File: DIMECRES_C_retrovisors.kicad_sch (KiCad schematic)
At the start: 65 parts, among them J10 Vbat, J2 DE9_Pins, J3 Conn_01x05_Pin, J4 Motor3, J6 Intermitente, J7 Calentador, J8 Motor2, J9 Motor1, Q1 DTC144E, Q2 DTC144E, Q3 DTC144E, SW1 SW_DPDT_G6S, U2 LM1117DT-ADJ, U3 LM2596S-ADJ, U4 L298N, U5 TJA1042T, U6 ADA4511-2, U7 PIC18F4480-IP, Y1 Crystal

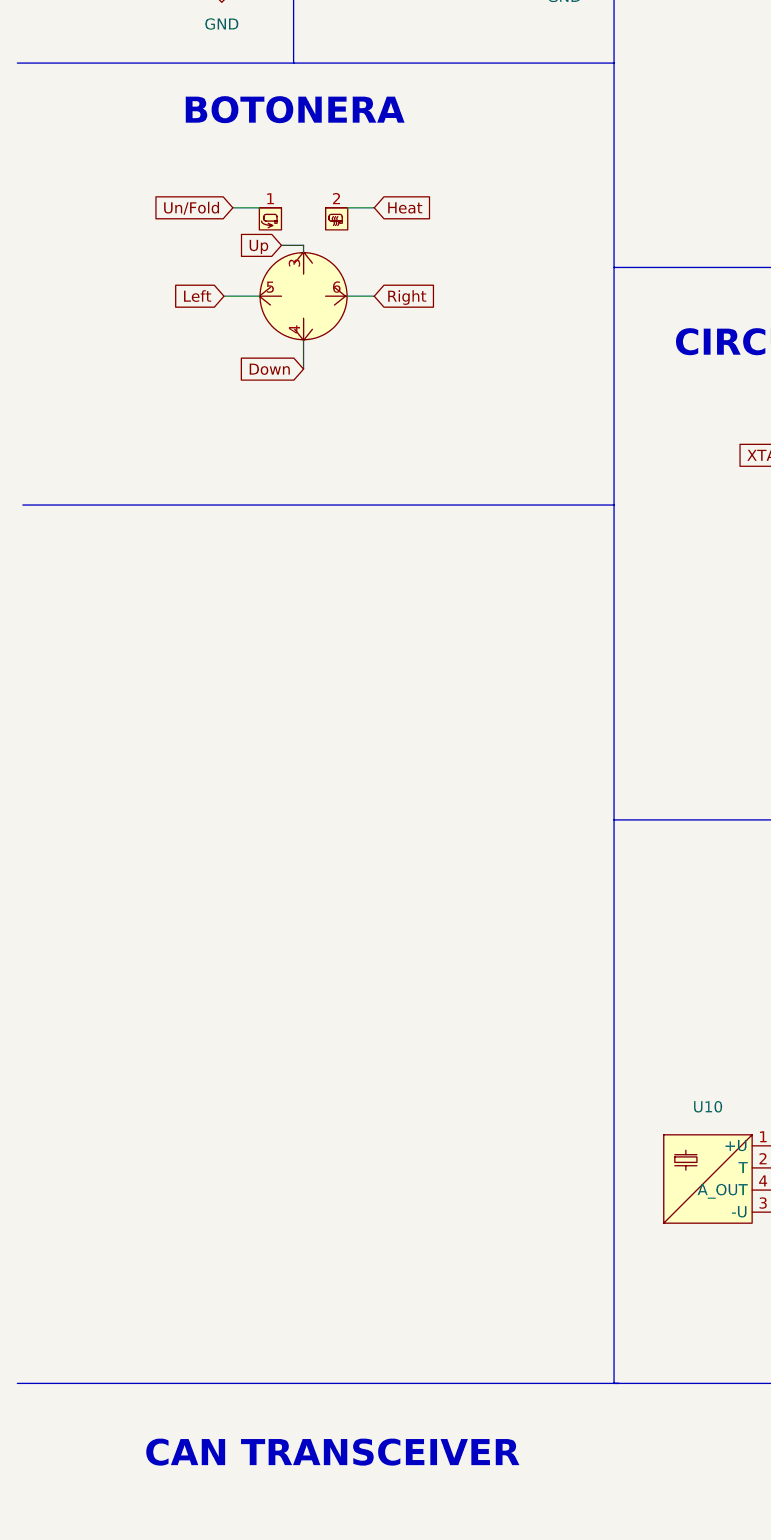
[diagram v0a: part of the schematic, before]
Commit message: Update DIMECRES_C_retrovisors.kicad_sch
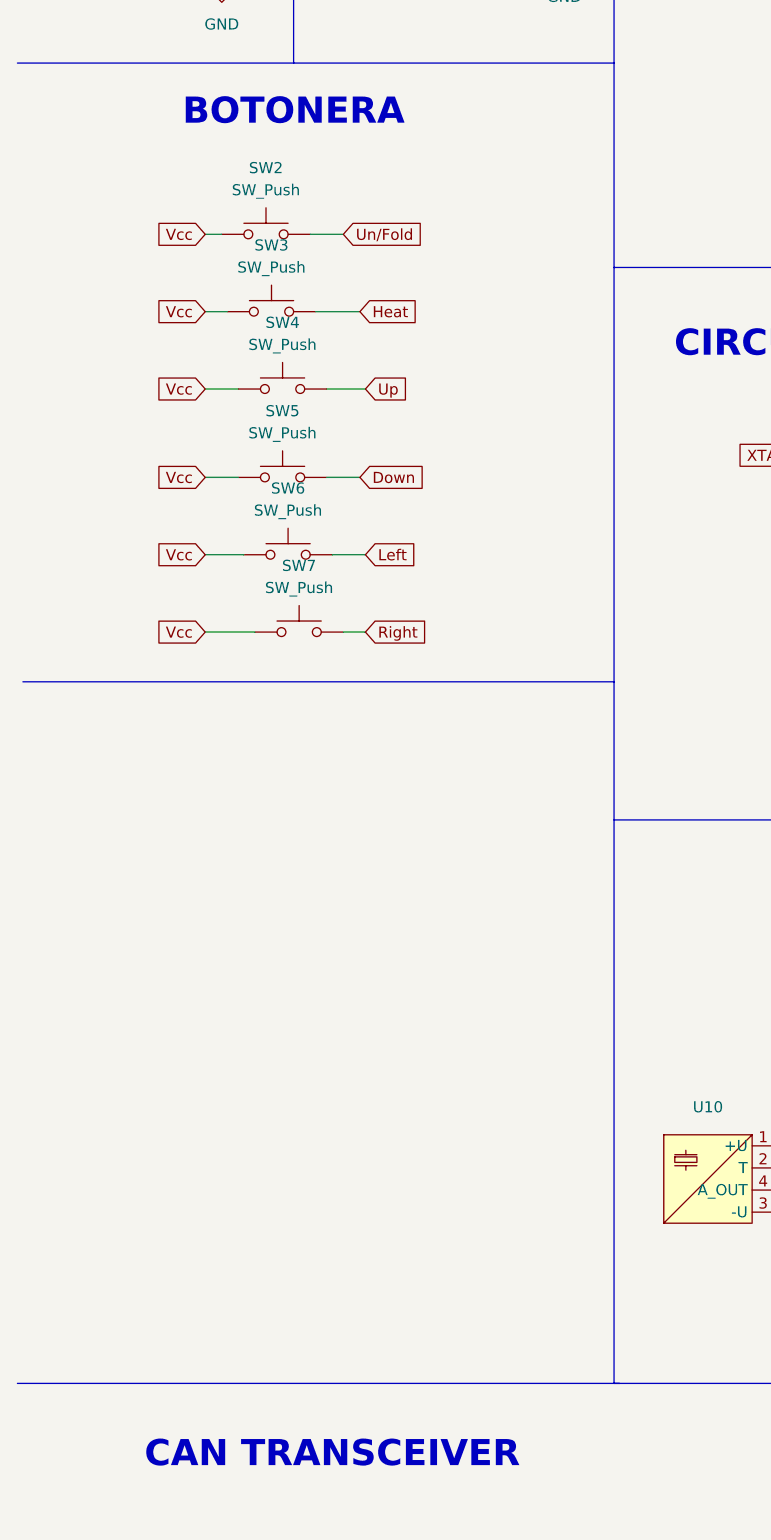
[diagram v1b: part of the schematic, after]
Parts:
- removed U1: ~, symbol PracticasKiCad:Botonera_Retrovisor
- added SW2, SW3, SW4, SW5, SW6, SW7: SW_Push, symbol Switch:SW_Push
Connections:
- net Down: now also SW5.2
- net Heat: now also SW3.2
- net Left: now also SW6.2
- net Right: now also SW7.2
- net Un/Fold: now also SW2.2
- net Up: now also SW4.2
- net Vcc: now also SW2.1, SW3.1, SW4.1, SW5.1, SW6.1, SW7.1
